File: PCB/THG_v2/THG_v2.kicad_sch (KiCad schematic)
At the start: 11 parts, among them J1 AM2315_Conn, J2 LCD_conn, J3 RTC_Conn, J4 SD_card_conn, J5 Screw_Terminal_01x02, U1 mini_esp32

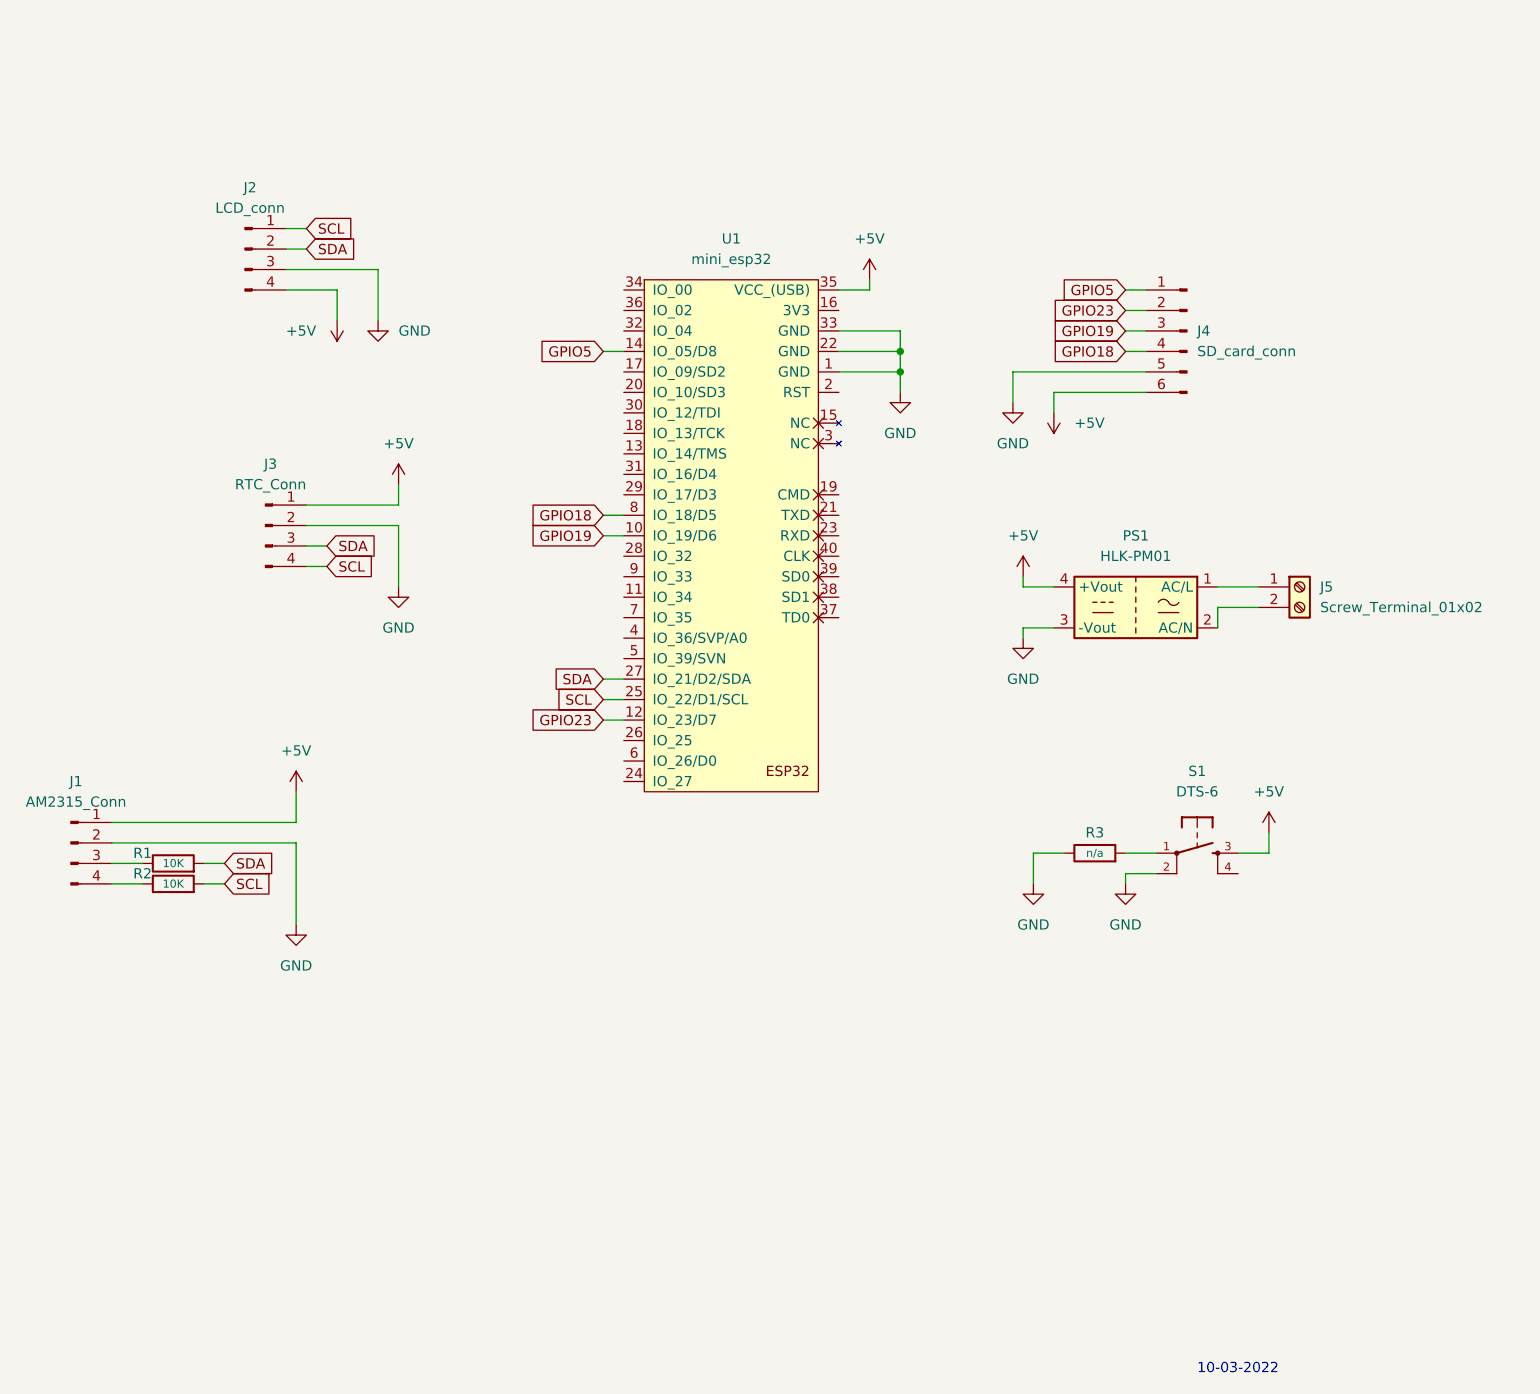
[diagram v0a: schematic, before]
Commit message: adding pcb pic
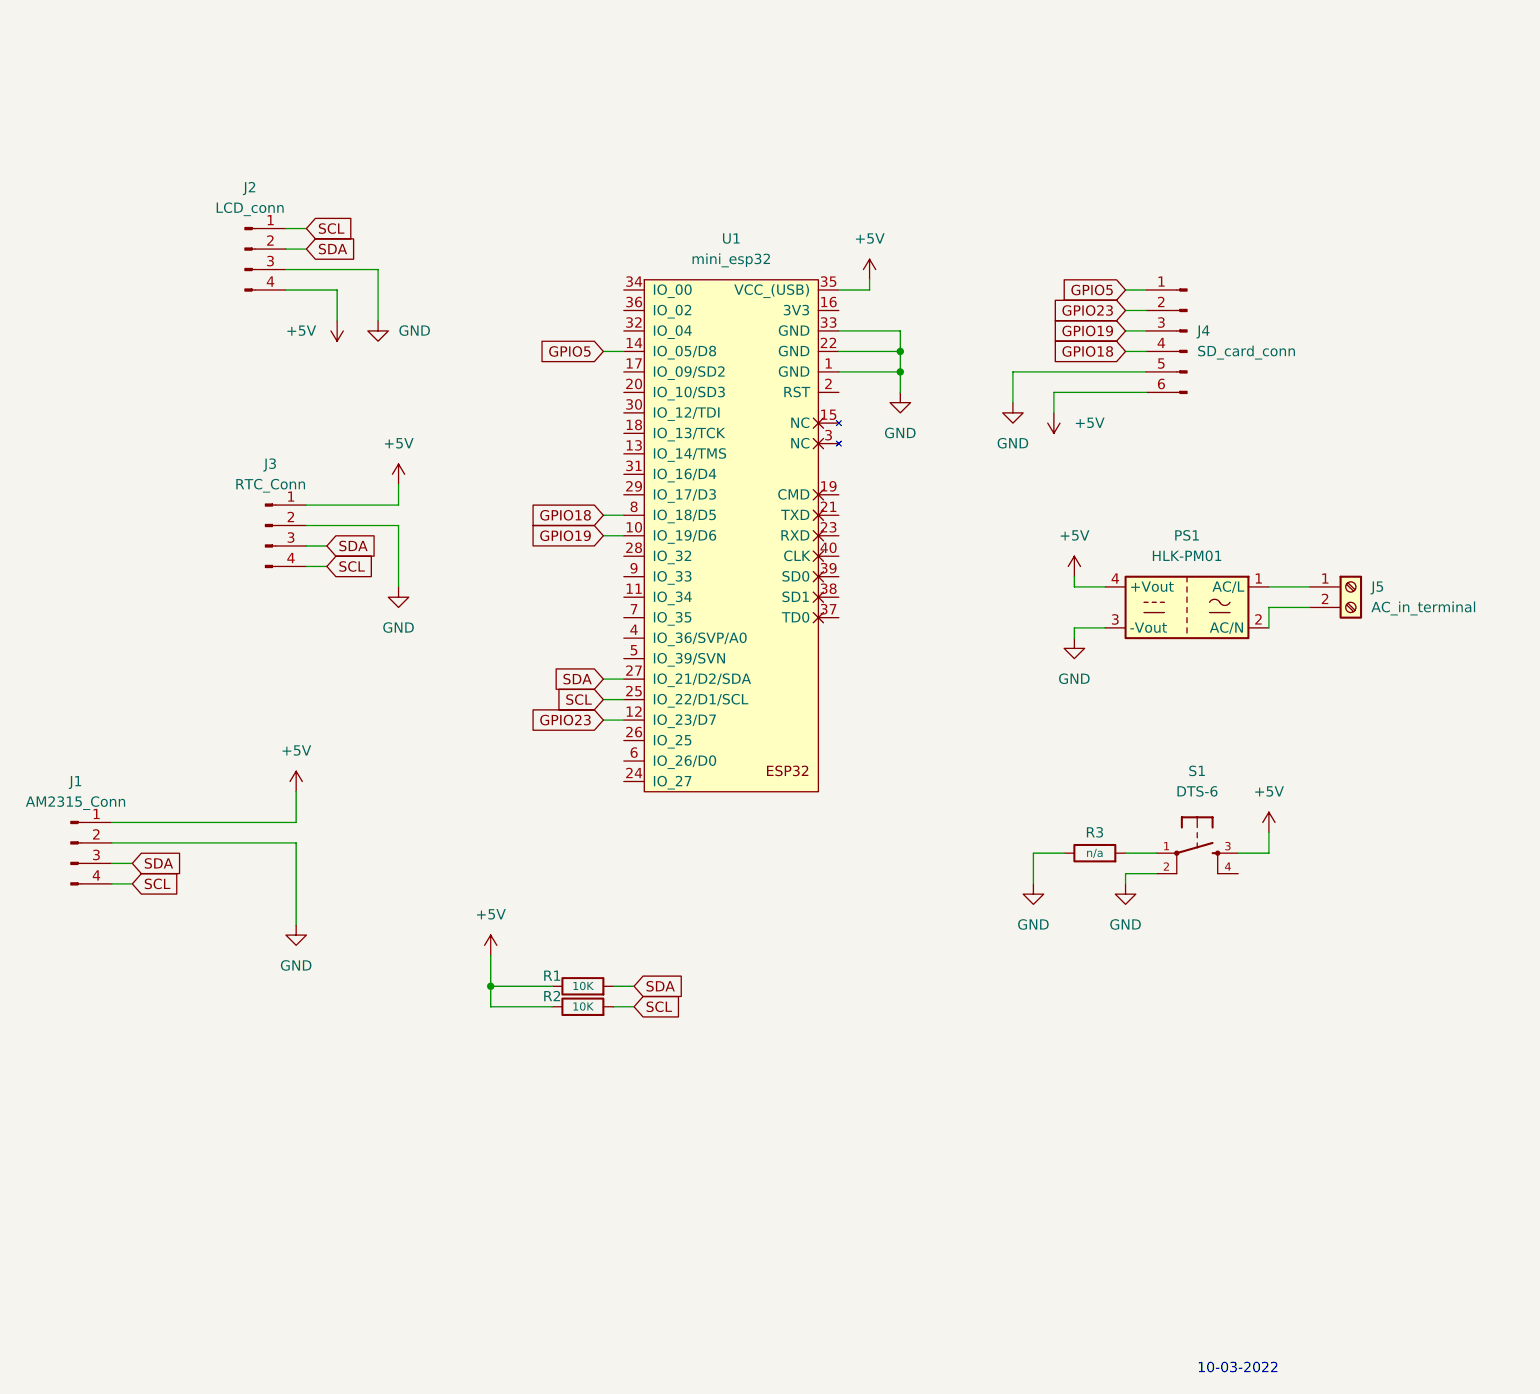
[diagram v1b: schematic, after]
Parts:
- J5: value Screw_Terminal_01x02 -> AC_in_terminal
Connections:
- net +5V: now also R1.1, R2.1
- net SCL: now also J1.4 (Pin_4)
- net SDA: now also J1.3 (Pin_3)
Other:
- moved on the sheet: J5, R1, R2

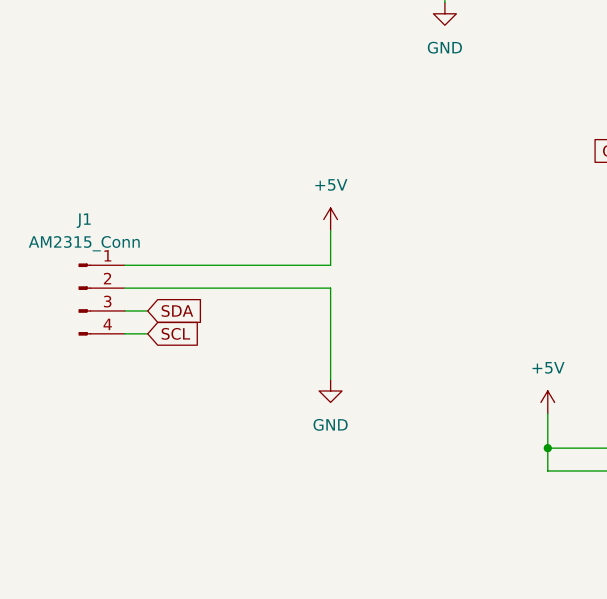
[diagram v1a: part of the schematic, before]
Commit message: rev
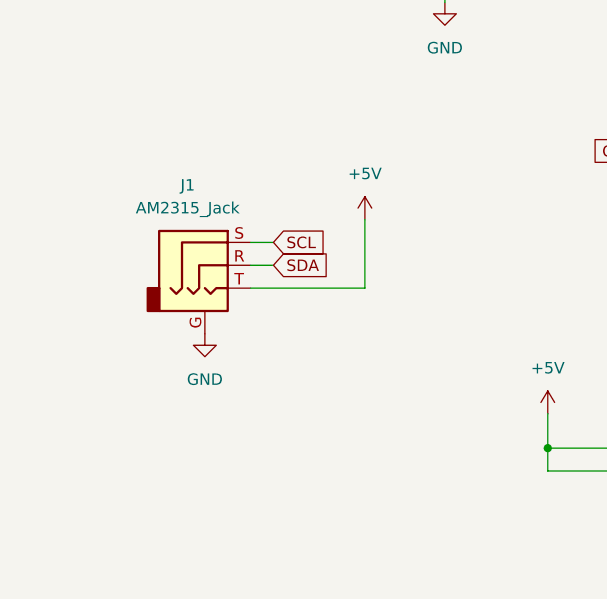
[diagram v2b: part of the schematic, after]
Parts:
- removed J1: AM2315_Conn, Connector_JST:JST_EH_B4B-EH-A_1x04_P2.50mm_Vertical, symbol Connector:Conn_01x04_Male
- added J1: AM2315_Jack, Lib_Kicad:TRRS-PJ-320A, symbol Connector:AudioJack3_Ground
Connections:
- net +5V: now also J1.T
- net GND: now also J1.G
- net SCL: now also J1.S
- net SDA: now also J1.R
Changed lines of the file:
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@@
-    (stroke (width 0) (type default) (color 0 0 0 0))
-  )
-  (wire (pts (xy 95.25 138.43) (xy 95.25 128.27))
-    (stroke (width 0) (type default) (color 0 0 0 0))
-  )
-  (wire (pts (xy 95.25 121.92) (xy 95.25 125.73))
     (stroke (width 0) (type default) (color 0 0 0 0))
   )
@@
     (stroke (width 0) (type default) (color 0 0 0 0))
   )
+  (wire (pts (xy 86.36 128.27) (xy 99.06 128.27))
+    (stroke (width 0) (type default) (color 0 0 0 0))
+  )
   (wire (pts (xy 215.9 129.54) (xy 212.09 129.54))
     (stroke (width 0) (type default) (color 0 0 0 0))
   )
-  (wire (pts (xy 74.93 133.35) (xy 72.39 133.35))
+  (wire (pts (xy 88.9 123.19) (xy 86.36 123.19))
     (stroke (width 0) (type default) (color 0 0 0 0))
   )
@@
     (stroke (width 0) (type default) (color 0 0 0 0))
   )
-  (wire (pts (xy 74.93 130.81) (xy 72.39 130.81))
+  (wire (pts (xy 88.9 125.73) (xy 86.36 125.73))
     (stroke (width 0) (type default) (color 0 0 0 0))
   )
@@
     (stroke (width 0) (type default) (color 0 0 0 0))
   )
-  (wire (pts (xy 95.25 128.27) (xy 72.39 128.27))
-    (stroke (width 0) (type default) (color 0 0 0 0))
-  )
   (wire (pts (xy 198.12 62.23) (xy 200.66 62.23))
     (stroke (width 0) (type default) (color 0 0 0 0))
@@
     (stroke (width 0) (type default) (color 0 0 0 0))
   )
+  (wire (pts (xy 99.06 128.27) (xy 99.06 120.65))
+    (stroke (width 0) (type default) (color 0 0 0 0))
+  )
   (wire (pts (xy 99.06 93.98) (xy 96.52 93.98))
-    (stroke (width 0) (type default) (color 0 0 0 0))
-  )
-  (wire (pts (xy 95.25 125.73) (xy 72.39 125.73))
     (stroke (width 0) (type default) (color 0 0 0 0))
   )
@@
     )
   )
-  (global_label "SDA" (shape input) (at 74.93 130.81 0) (fields_autoplaced)
+  (global_label "SDA" (shape input) (at 88.9 125.73 0) (fields_autoplaced)
     (effects (font (size 1.27 1.27)) (justify left))
-    (property "Intersheet References" "${INTERSHEET_REFS}" (id 0) (at 80.9112 130.7306 0)
+    (property "Intersheet References" "${INTERSHEET_REFS}" (id 0) (at 94.8812 125.8094 0)
       (effects (font (size 1.27 1.27)) (justify left) hide)
     )
@@
     )
   )
-  (global_label "SCL" (shape input) (at 74.93 133.35 0) (fields_autoplaced)
+  (global_label "SCL" (shape input) (at 88.9 123.19 0) (fields_autoplaced)
     (effects (font (size 1.27 1.27)) (justify left))
-    (property "Intersheet References" "${INTERSHEET_REFS}" (id 0) (at 80.8507 133.2706 0)
+    (property "Intersheet References" "${INTERSHEET_REFS}" (id 0) (at 94.8207 123.2694 0)
       (effects (font (size 1.27 1.27)) (justify left) hide)
     )
@@
     (pin "1")
   )
-  (symbol (lib_id "Connector:Conn_01x04_Male") (at 67.31 128.27 0) (unit 1)
-    (in_bom yes) (on_board yes) (fields_autoplaced)
-    (property "Reference" "J1" (id 0) (at 67.945 120.65 0))
-    (property "Value" "AM2315_Conn" (id 1) (at 67.945 123.19 0))
-    (property "Footprint" "Connector_JST:JST_EH_B4B-EH-A_1x04_P2.50mm_Vertical" (id 2) (at 67.31 128.27 0)
-      (effects (font (size 1.27 1.27)) hide)
-    )
-    (property "Datasheet" "~" (id 3) (at 67.31 128.27 0)
-      (effects (font (size 1.27 1.27)) hide)
-    )
-    (pin "1")
-    (pin "2")
-    (pin "3")
-    (pin "4")
+  (symbol (lib_id "Connector:AudioJack3_Ground") (at 81.28 125.73 0) (unit 1)
+    (in_bom yes) (on_board yes) (fields_autoplaced)
+    (property "Reference" "J1" (id 0) (at 79.375 116.84 0))
+    (property "Value" "AM2315_Jack" (id 1) (at 79.375 119.38 0))
+    (property "Footprint" "Lib_Kicad:TRRS-PJ-320A" (id 2) (at 81.28 125.73 0)
+      (effects (font (size 1.27 1.27)) hide)
+    )
+    (property "Datasheet" "~" (id 3) (at 81.28 125.73 0)
+      (effects (font (size 1.27 1.27)) hide)
+    )
+    (pin "G")
+    (pin "R")
+    (pin "S")
+    (pin "T")
   )
   (symbol (lib_id "DTS-6:DTS-6") (at 207.01 129.54 270) (unit 1)
@@
     (pin "1")
   )
-  (symbol (lib_id "power:+5V") (at 95.25 121.92 0) (unit 1)
-    (in_bom yes) (on_board yes) (fields_autoplaced)
-    (property "Reference" "#PWR0105" (id 0) (at 95.25 125.73 0)
-      (effects (font (size 1.27 1.27)) hide)
-    )
-    (property "Value" "+5V" (id 1) (at 95.25 116.84 0))
-    (property "Footprint" "" (id 2) (at 95.25 121.92 0)
-      (effects (font (size 1.27 1.27)) hide)
-    )
-    (property "Datasheet" "" (id 3) (at 95.25 121.92 0)
+  (symbol (lib_id "power:+5V") (at 99.06 120.65 0) (mirror y) (unit 1)
+    (in_bom yes) (on_board yes) (fields_autoplaced)
+    (property "Reference" "#PWR0105" (id 0) (at 99.06 124.46 0)
+      (effects (font (size 1.27 1.27)) hide)
+    )
+    (property "Value" "+5V" (id 1) (at 99.06 115.57 0))
+    (property "Footprint" "" (id 2) (at 99.06 120.65 0)
+      (effects (font (size 1.27 1.27)) hide)
+    )
+    (property "Datasheet" "" (id 3) (at 99.06 120.65 0)
       (effects (font (size 1.27 1.27)) hide)
     )
@@
   (symbol (lib_id "power:+5V") (at 119.38 142.24 0) (unit 1)
     (in_bom yes) (on_board yes) (fields_autoplaced)
-    (property "Reference" "#PWR?" (id 0) (at 119.38 146.05 0)
+    (property "Reference" "#PWR0116" (id 0) (at 119.38 146.05 0)
       (effects (font (size 1.27 1.27)) hide)
     )
@@
     (pin "1")
   )
-  (symbol (lib_id "power:GND") (at 95.25 138.43 0) (unit 1)
-    (in_bom yes) (on_board yes) (fields_autoplaced)
-    (property "Reference" "#PWR0106" (id 0) (at 95.25 144.78 0)
-      (effects (font (size 1.27 1.27)) hide)
-    )
-    (property "Value" "GND" (id 1) (at 95.25 143.51 0))
-    (property "Footprint" "" (id 2) (at 95.25 138.43 0)
-      (effects (font (size 1.27 1.27)) hide)
-    )
-    (property "Datasheet" "" (id 3) (at 95.25 138.43 0)
+  (symbol (lib_id "power:GND") (at 81.28 133.35 0) (unit 1)
+    (in_bom yes) (on_board yes) (fields_autoplaced)
+    (property "Reference" "#PWR0106" (id 0) (at 81.28 139.7 0)
+      (effects (font (size 1.27 1.27)) hide)
+    )
+    (property "Value" "GND" (id 1) (at 81.28 138.43 0))
+    (property "Footprint" "" (id 2) (at 81.28 133.35 0)
+      (effects (font (size 1.27 1.27)) hide)
+    )
+    (property "Datasheet" "" (id 3) (at 81.28 133.35 0)
       (effects (font (size 1.27 1.27)) hide)
     )
@@
     )
     (path "/50c1423a-2336-485b-a1eb-eea3967751f9"
-      (reference "#PWR?") (unit 1) (value "+5V") (footprint "")
-    )
-    (path "/27d7923d-62c0-4fe7-8bd6-2b6190754bc6"
-      (reference "J1") (unit 1) (value "AM2315_Conn") (footprint "Connector_JST:JST_EH_B4B-EH-A_1x04_P2.50mm_Vertical")
+      (reference "#PWR0116") (unit 1) (value "+5V") (footprint "")
+    )
+    (path "/1e362064-1c5c-469c-8576-28390879d190"
+      (reference "J1") (unit 1) (value "AM2315_Jack") (footprint "Lib_Kicad:TRRS-PJ-320A")
     )
     (path "/eacfccdb-496f-4d23-be5f-1e7301d4a980"
